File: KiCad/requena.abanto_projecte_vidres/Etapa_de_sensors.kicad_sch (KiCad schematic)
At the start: 18 parts, among them SW1 SW_Omron_B3FS, SW2 SW_Push_SPDT, SW3 SW_Omron_B3FS, SW4 SW_Omron_B3FS, SW5 SW_Omron_B3FS, U1 PN5120A0HN1, U2 MCP6001-OT, Y1 Crystal

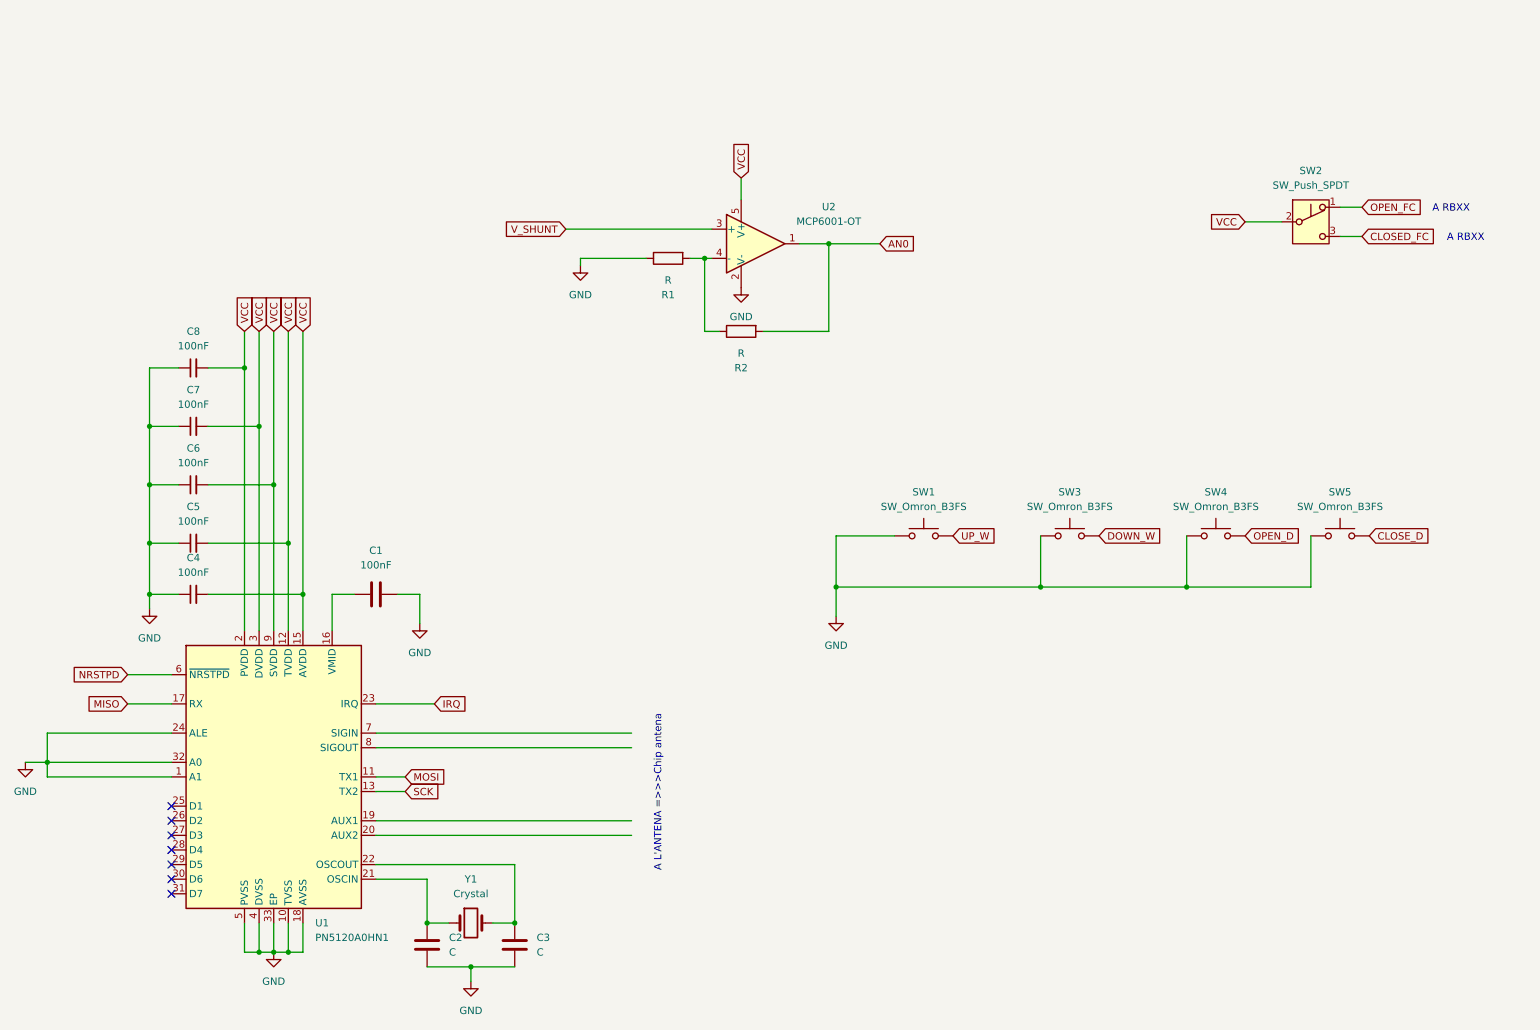
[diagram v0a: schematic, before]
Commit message: cambios de clase
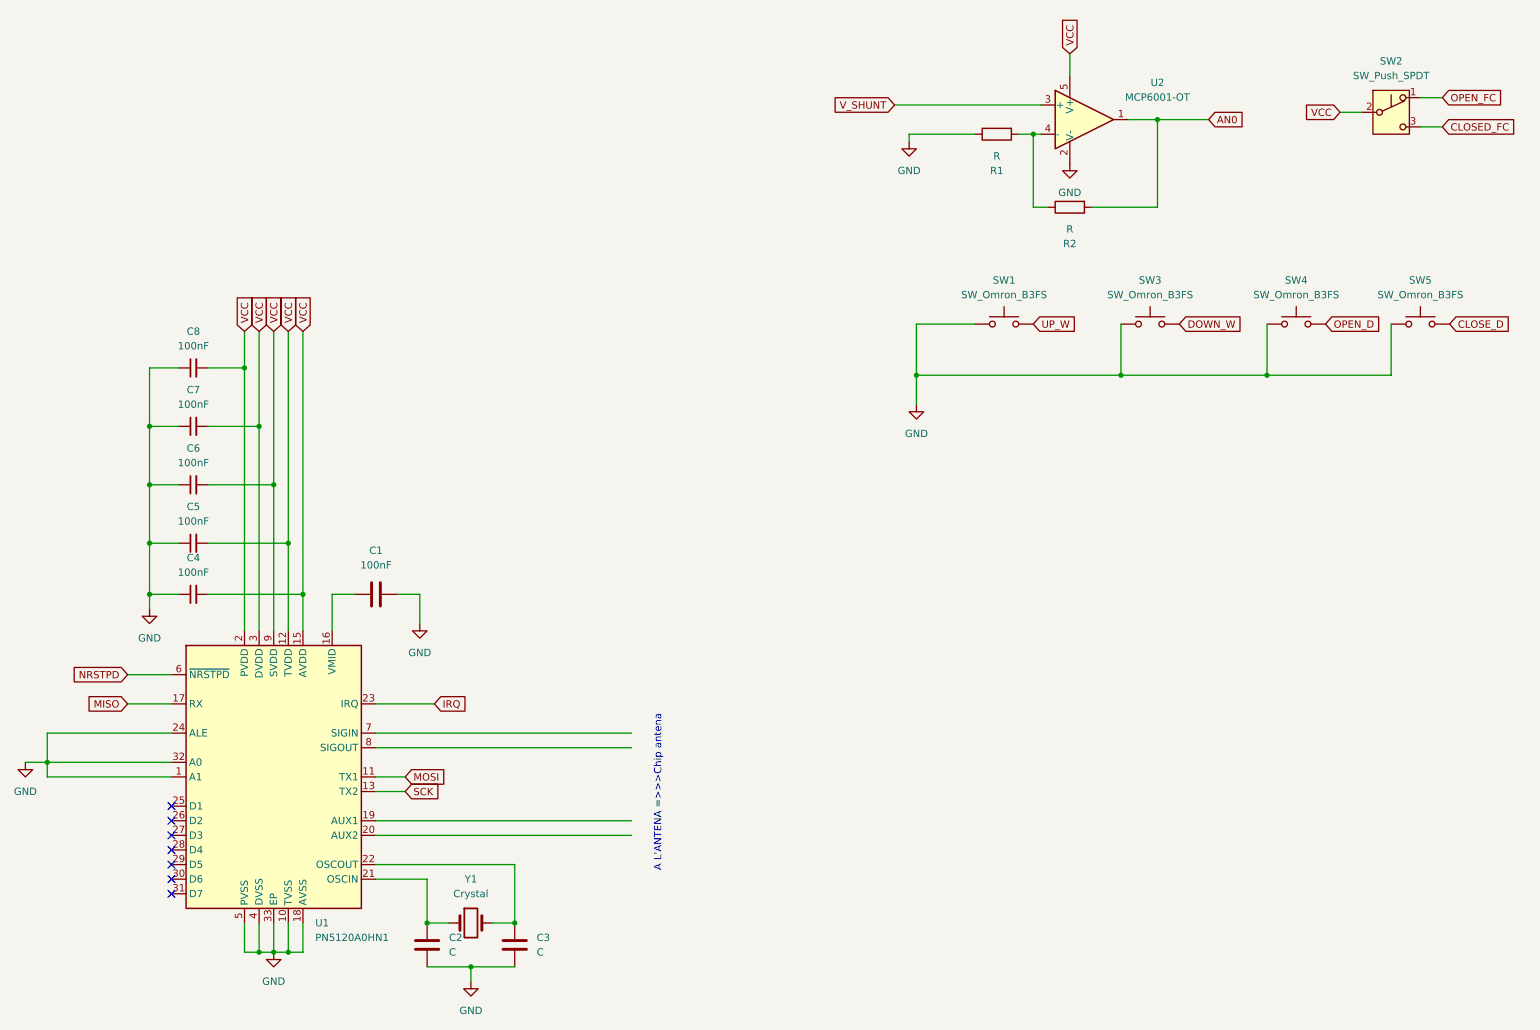
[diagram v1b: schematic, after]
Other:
- note removed: "A RBXX"
- moved on the sheet: R1, R2, SW1, SW2, SW3, SW4, SW5, U2
